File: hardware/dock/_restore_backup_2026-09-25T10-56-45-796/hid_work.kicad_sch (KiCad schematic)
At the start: 15 parts, among them J3 Conn_01x05_Pin, J4 L-KLS1-5416-L1-01-R, U5 TPD4E1U06DBVR

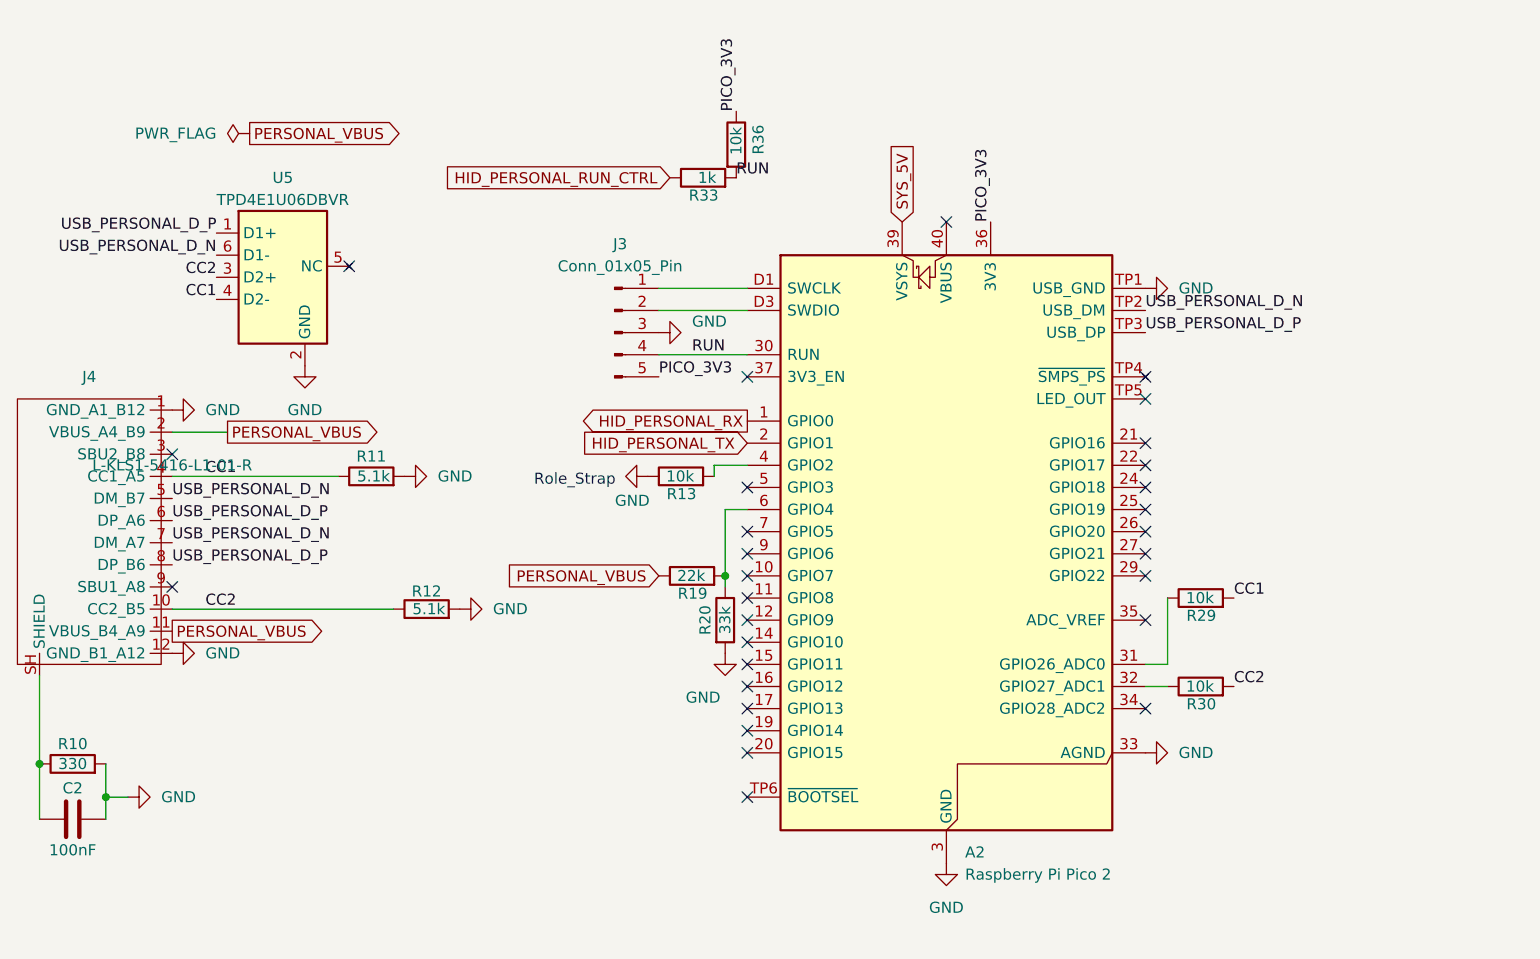
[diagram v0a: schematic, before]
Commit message: a small backup commit
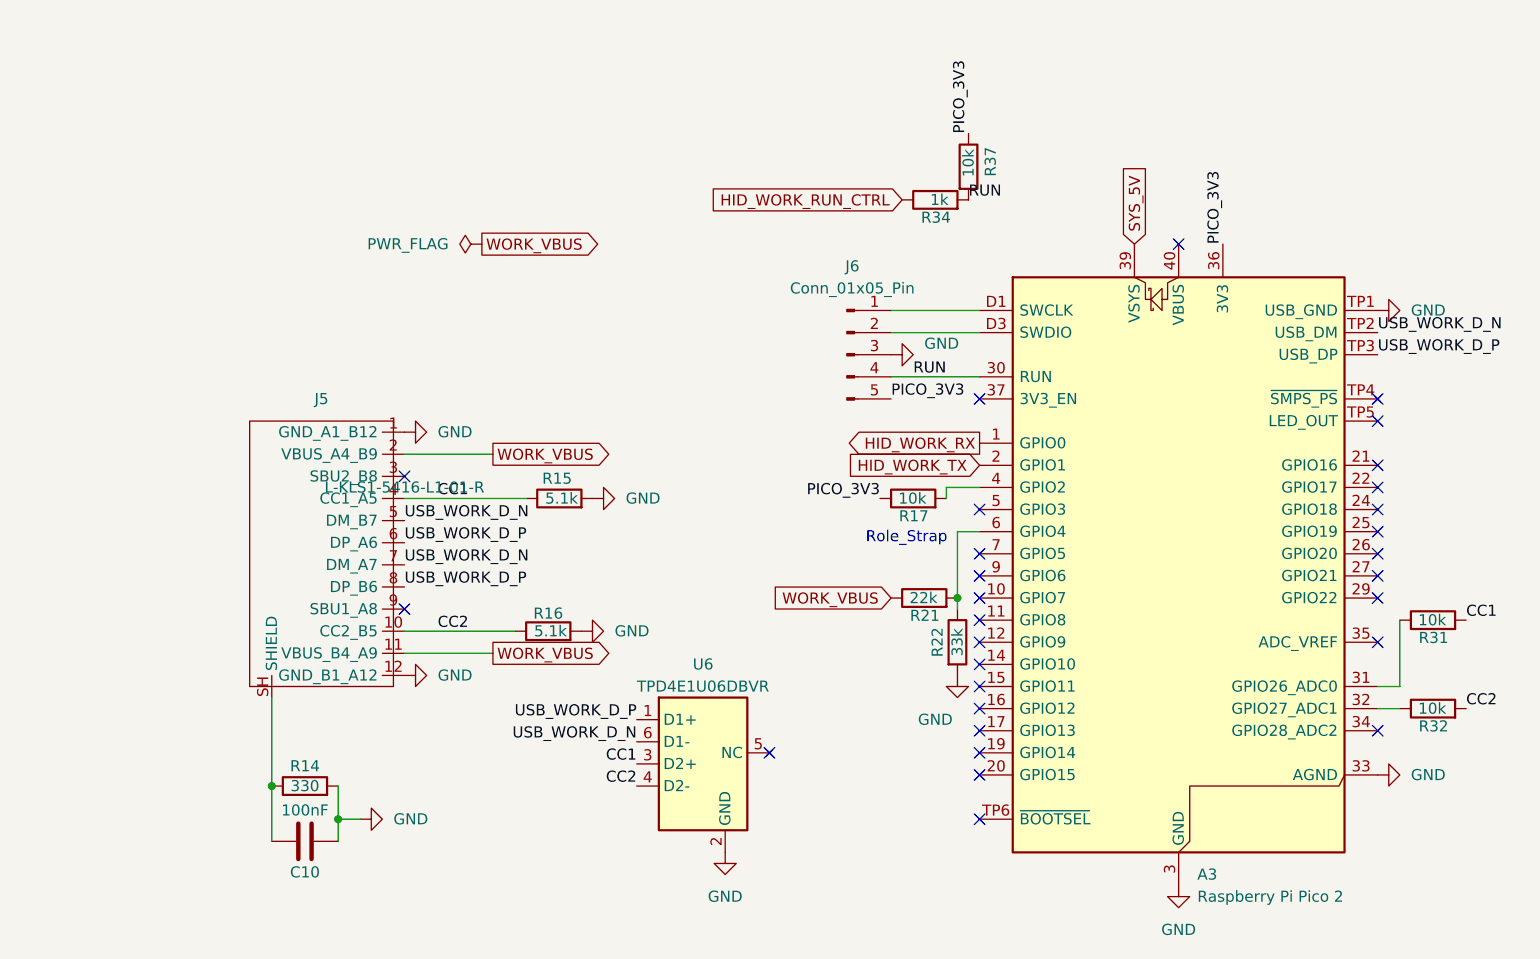
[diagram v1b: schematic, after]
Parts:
- removed A2: Raspberry Pi Pico 2, dock:RaspberryPi_Pico2_Socket_Pogo, symbol MCU_Module:RaspberryPi_Pico_Extensive
- removed C2: 100nF, Capacitor_SMD:C_0805_2012Metric_Pad1.18x1.45mm_HandSolder, symbol Device:C
- removed J3: Conn_01x05_Pin, Connector_PinHeader_2.54mm:PinHeader_1x05_P2.54mm_Vertical, symbol Connector:Conn_01x05_Pin
- removed J4: L-KLS1-5416-L1-01-R, dock:KLS L-KLS1-5416-L1-01-R, symbol dock_custom:KLS_L-KLS1-5416-L1-01-R
- removed R10: 330, Resistor_SMD:R_0805_2012Metric_Pad1.20x1.40mm_HandSolder, symbol Device:R
- removed R11, R12: 5.1k, Resistor_SMD:R_0805_2012Metric_Pad1.20x1.40mm_HandSolder, symbol Device:R
- removed R13, R29, R30, R36: 10k, Resistor_SMD:R_0805_2012Metric_Pad1.20x1.40mm_HandSolder, symbol Device:R
- removed R19: 22k, Resistor_SMD:R_0805_2012Metric_Pad1.20x1.40mm_HandSolder, symbol Device:R
- removed R20: 33k, Resistor_SMD:R_0805_2012Metric_Pad1.20x1.40mm_HandSolder, symbol Device:R
- removed R33: 1k, Resistor_SMD:R_0805_2012Metric_Pad1.20x1.40mm_HandSolder, symbol Device:R
- removed U5: TPD4E1U06DBVR, Package_TO_SOT_SMD:SOT-23-6, symbol dock_custom:TPD4E1U06DBV
- added A3: Raspberry Pi Pico 2, dock:RaspberryPi_Pico2_Socket_Pogo, symbol MCU_Module:RaspberryPi_Pico_Extensive
- added C10: 100nF, Capacitor_SMD:C_0805_2012Metric_Pad1.18x1.45mm_HandSolder, symbol Device:C
- added J5: L-KLS1-5416-L1-01-R, dock:KLS L-KLS1-5416-L1-01-R, symbol dock_custom:KLS_L-KLS1-5416-L1-01-R
- added J6: Conn_01x05_Pin, Connector_PinHeader_2.54mm:PinHeader_1x05_P2.54mm_Vertical, symbol Connector:Conn_01x05_Pin
- added R14: 330, Resistor_SMD:R_0805_2012Metric_Pad1.20x1.40mm_HandSolder, symbol Device:R
- added R15, R16: 5.1k, Resistor_SMD:R_0805_2012Metric_Pad1.20x1.40mm_HandSolder, symbol Device:R
- added R17, R31, R32, R37: 10k, Resistor_SMD:R_0805_2012Metric_Pad1.20x1.40mm_HandSolder, symbol Device:R
- added R21: 22k, Resistor_SMD:R_0805_2012Metric_Pad1.20x1.40mm_HandSolder, symbol Device:R
- added R22: 33k, Resistor_SMD:R_0805_2012Metric_Pad1.20x1.40mm_HandSolder, symbol Device:R
- added R34: 1k, Resistor_SMD:R_0805_2012Metric_Pad1.20x1.40mm_HandSolder, symbol Device:R
- added U6: TPD4E1U06DBVR, Package_TO_SOT_SMD:SOT-23-6, symbol dock_custom:TPD4E1U06DBV
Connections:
- net CC1: now also J5.4 (CC1_A5), R15.1, R31.2, U6.3 (D2+)
- net CC2: now also J5.10 (CC2_B5), R16.1, R32.2, U6.4 (D2-)
- net GND: now also A3.13 (GND), A3.18 (GND), A3.23 (GND), A3.28 (GND), A3.3 (GND), A3.33 (AGND), A3.38 (GND), A3.8 (GND), A3.D2 (GND), A3.TP1 (USB_GND), C10.2, J5.1 (GND_A1_B12), J5.12 (GND_B1_A12), J6.3 (Pin_3), R14.2, R15.2, R16.2, R22.2, U6.2 (GND)
- net PICO_3V3: now also A3.36 (3V3), J6.5 (Pin_5), R17.1, R37.1
- net RUN: now also A3.30 (RUN), J6.4 (Pin_4), R34.2, R37.2
- net SYS_5V: now also A3.39 (VSYS)
- new net: A3.D1 (SWCLK), J6.1 (Pin_1)
- new net: A3.D3 (SWDIO), J6.2 (Pin_2)
- new net: C10.1, J5.SH (SHIELD), R14.1
- new net: A3.6 (GPIO4), R21.2, R22.1
- new net: A3.31 (GPIO26_ADC0), R31.1
- new net: A3.32 (GPIO27_ADC1), R32.1
- new net: A3.4 (GPIO2), R17.2
- new net HID_WORK_RUN_CTRL: R34.1
- new net HID_WORK_RX: A3.1 (GPIO0)
- new net HID_WORK_TX: A3.2 (GPIO1)
- new net USB_WORK_D_N: A3.TP2 (USB_DM), J5.5 (DM_B7), J5.7 (DM_A7), U6.6 (D1-)
- new net USB_WORK_D_P: A3.TP3 (USB_DP), J5.6 (DP_A6), J5.8 (DP_B6), U6.1 (D1+)
- new net WORK_VBUS: J5.11 (VBUS_B4_A9), J5.2 (VBUS_A4_B9), R21.1
